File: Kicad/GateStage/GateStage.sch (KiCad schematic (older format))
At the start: 5 parts

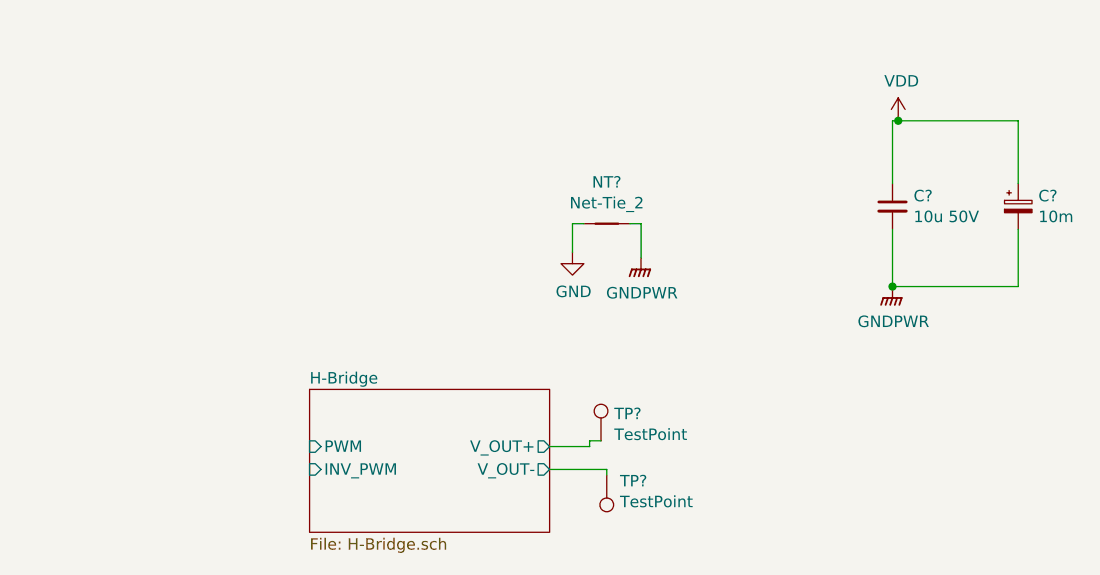
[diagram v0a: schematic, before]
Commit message: Gate Drive Board V 1
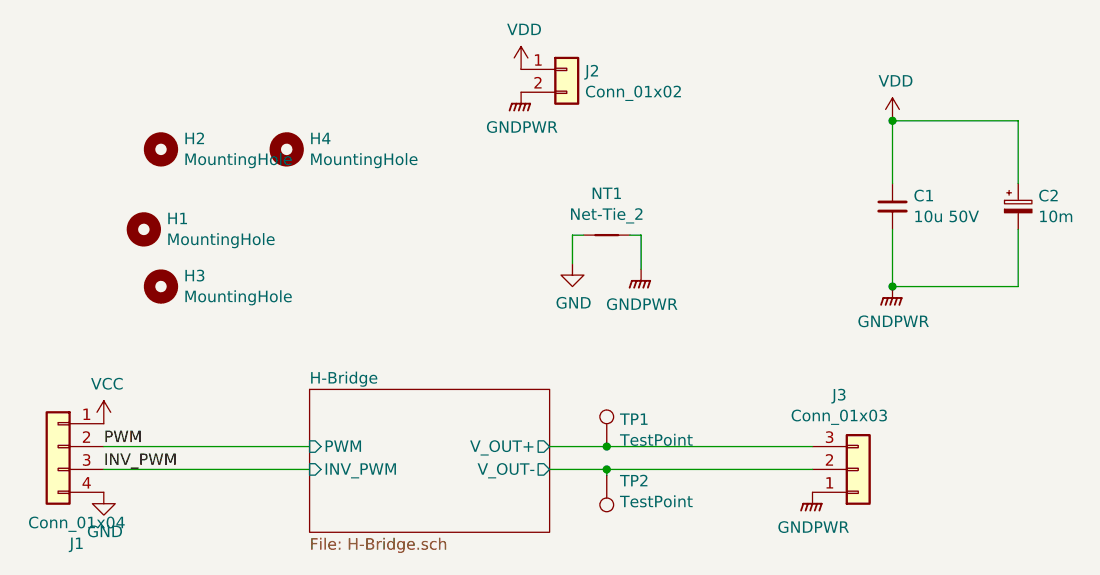
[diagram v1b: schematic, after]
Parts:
- added H1, H2, H3, H4: MountingHole, MountingHole:MountingHole_3.2mm_M3_ISO14580_Pad, symbol Mechanical:MountingHole
- added J1: Conn_01x04, TerminalBlock:TerminalBlock_bornier-4_P5.08mm, symbol Connector_Generic:Conn_01x04
- added J2: Conn_01x02, TerminalBlock:TerminalBlock_bornier-2_P5.08mm, symbol Connector_Generic:Conn_01x02
- added J3: Conn_01x03, TerminalBlock:TerminalBlock_bornier-3_P5.08mm, symbol Connector_Generic:Conn_01x03
- TP1, TP2: renamed from TP?; footprint (none) -> TestPoint:TestPoint_Pad_D2.0mm
- gave numbers to parts that had none: 3
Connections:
- net GND: now also J1.4 (Pin_4)
- net GNDPWR: now also J2.2 (Pin_2), J3.1 (Pin_1)
- net H-Bridge/V_OUT+: now also J3.3 (Pin_3)
- net H-Bridge/V_OUT-: now also J3.2 (Pin_2)
- net VDD: now also J2.1 (Pin_1)
- new net INV_PWM: J1.3 (Pin_3)
- new net PWM: J1.2 (Pin_2)
- new net VCC: J1.1 (Pin_1)
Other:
- moved on the sheet: NT1, TP1
